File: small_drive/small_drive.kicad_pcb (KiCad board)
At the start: 2 copper layers, 83.8 x 71.8 mm, 146 parts, among them CON1 BARREL_JACK, J1 DB9, M1 SiR826DP, M2 SiR826DP, M3 SiR826DP, M4 SiR826DP, M5 SiR826DP, M6 SiR826DP, M7 SiR826DP, P1 CONN_01X04, P10 CONN_01X02, P11 CONN_01X02, P12 CONN_01X02, P13 CONN_01X04, P14 CONN_01X02, P2 CONN_01X04, P3 CONN_01X06, P4 CONN_01X08, P5 CONN_01X02, P6 CONN_01X02, P7 CONN_01X02, P8 CONN_01X02, P9 CONN_01X04, U1 STM32F334K8, U10 LM5106, U11 ACS711ELCTR-25AB-T, U12 ACS711ELCTR-25AB-T, U13 ACS711ELCTR-25AB-T, U14 STM32F030F4P6TR, U15 LTC2850, U16 LIS3LV02DQ, U17 STM32F030F4P6TR, U18 LTC2850, U19 LIS3LV02DQ, U2 OKR_T3, U20 DS28CM00, U21 DS28CM00, U22 TL431, U23 LT3012, U24 STM32F030F4P6TR, U25 MC33074DTBR2, U3 LTC2850, U4 LTC2850, U5 LTC2850, U6 LT1764EQ, U7 MC33074DTBR2, U8 LM5106, U9 LM5106, Y1 Crystal

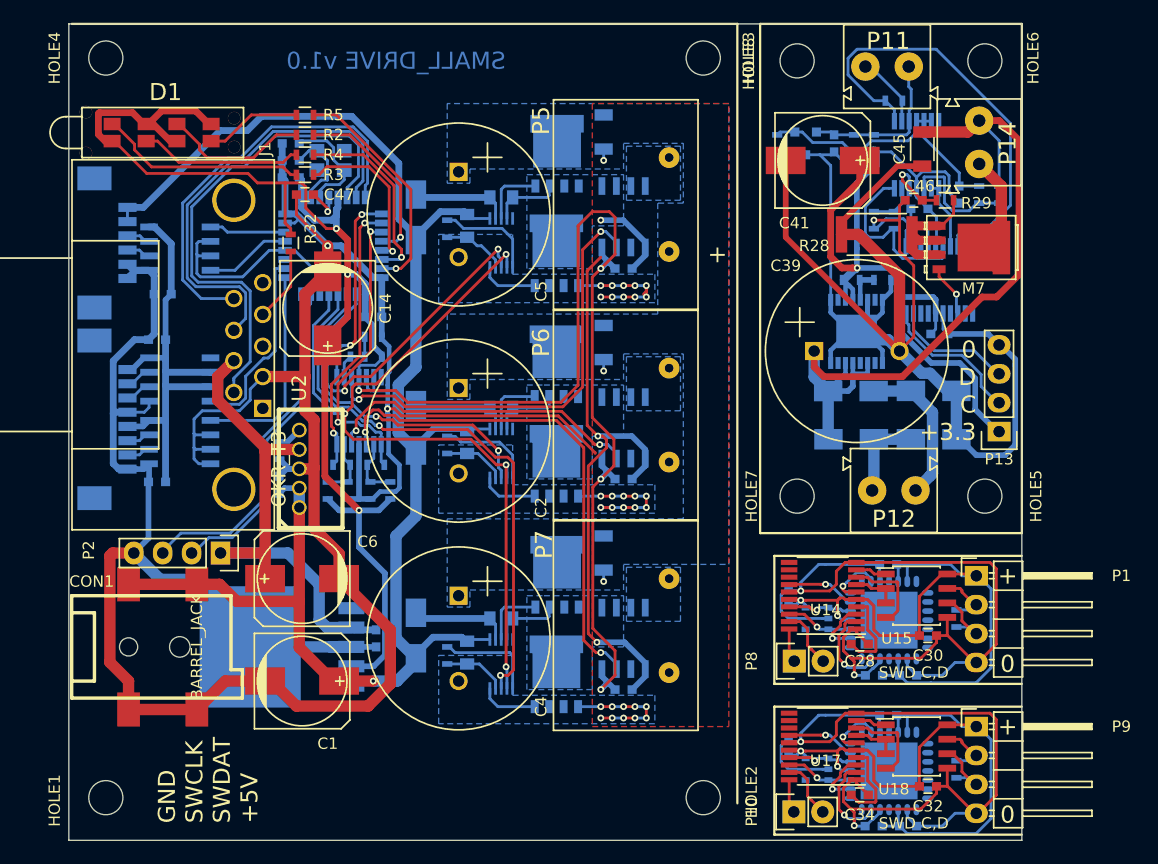
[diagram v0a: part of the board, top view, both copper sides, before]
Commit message: PCB ordered
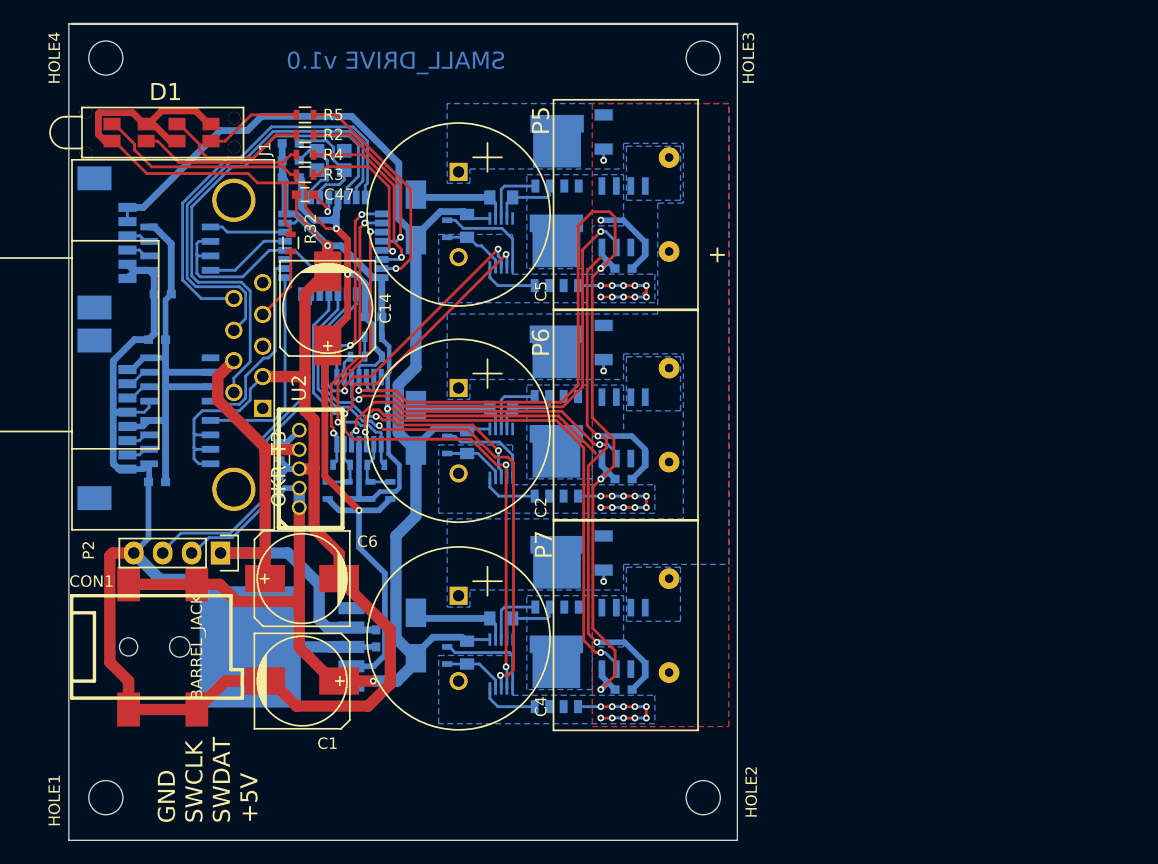
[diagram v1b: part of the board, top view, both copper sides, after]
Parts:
- removed C10, C11, C28, C29, C30, C31, C32, C33, C34, C35, C36, C37, C38, C40, C42, C43, C44: 100nF, Capacitors_SMD:C_0603
- removed C39: 470uF/63V, Capacitors_ThroughHole:C_Radial_D16_L25_P7.5
- removed C41: 100uF/35V, Capacitors_SMD:c_elec_8x10.5
- removed C45: 1uF/100V, Capacitors_SMD:C_1206
- removed C46: C, Capacitors_SMD:C_0603
- removed D5, D6, D7, D8: STPS2150A, Diodes_SMD:SMA_Standard
- removed HOLE5, HOLE6, HOLE7, HOLE8: HOLE, Mounting_Holes:MountingHole_3mm
- removed M7: SiR826DP, 00_Passives:SOT-669_GDS
- removed P1, P9: CONN_01X04, Pin_Headers:Pin_Header_Angled_1x04
- removed P10, P8: CONN_01X02, Pin_Headers:Pin_Header_Straight_1x02
- removed P11, P12, P14: CONN_01X02, 00_Passives:Wiecon_25.197.0253.0
- removed P13: CONN_01X04, Pin_Headers:Pin_Header_Straight_1x04
- removed R18, R19: R, Resistors_SMD:R_0603
- removed R20: 1.5k, Resistors_SMD:R_0603
- removed R21: 300, Resistors_SMD:R_0603
- removed R22: 910, Resistors_SMD:R_0603
- removed R23, R29, R30, R31: 1k, Resistors_SMD:R_0603
- removed R24: 3.0k, Resistors_SMD:R_0603
- removed R25: 1.8k, Resistors_SMD:R_0603
- removed R26: 51k, Resistors_SMD:R_0603
- removed R27: 2.2k, Resistors_SMD:R_0603
- removed R28: R, Resistors_SMD:R_2512
- removed U14, U17, U24: STM32F030F4P6TR, Housings_SSOP:TSSOP-20_4.4x6.5mm_Pitch0.65mm
- removed U15, U18: LTC2850, Housings_SOIC:SOIC-8_3.9x4.9mm_Pitch1.27mm
- removed U16, U19: LIS3LV02DQ, Housings_DFN_QFN:QFN-28-1EP_7x7mm_Pitch0.8mm
- removed U20, U21: DS28CM00, 00_Passives:SOT23_5
- removed U22: TL431, TO_SOT_Packages_SMD:SOT-23
- removed U23: LT3012, Housings_SSOP:TSSOP-16-1EP_4.4x5mm_Pitch0.65mm
- removed U25: MC33074DTBR2, Housings_SSOP:TSSOP-14_4.4x5mm_Pitch0.65mm
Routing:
- net /pomp/Vss: track 169.7 -> 0.00 mm, vias 1 -> 0
- net /pomp/Vdd: track 81.8 -> 0.00 mm, vias 1 -> 0
- net /g_sensor2/Vss: track 79.3 -> 0.00 mm, vias 2 -> 0
- net /g_sensor1/Vss: track 79.3 -> 0.00 mm, vias 2 -> 0
- net /pomp/Vpower: track 69.4 -> 0.00 mm
- net /g_sensor1/Vdd: track 59.6 -> 0.00 mm, vias 2 -> 0
- net /g_sensor2/Vdd: track 59.6 -> 0.00 mm, vias 2 -> 0
- net /pomp/MAINS: track 39.0 -> 0.00 mm
- net /pomp/CURRENT: track 16.0 -> 0.00 mm
- net Net-(C38-Pad1): track 14.3 -> 0.00 mm
- net Net-(D7-PadA): track 13.8 -> 0.00 mm
- net /pomp/SWCLK: track 12.8 -> 0.00 mm
- net Net-(M7-PadS): track 12.5 -> 0.00 mm
- net /pomp/SWDIO: track 10.6 -> 0.00 mm
- net Net-(R26-Pad2): track 10.4 -> 0.00 mm
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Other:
- board size 83.8 x 71.8 mm -> 58.8 x 71.8 mm
- board text removed: "0"
- board text removed: "0 D C +3.3"
- board text removed: "SWD C,D"

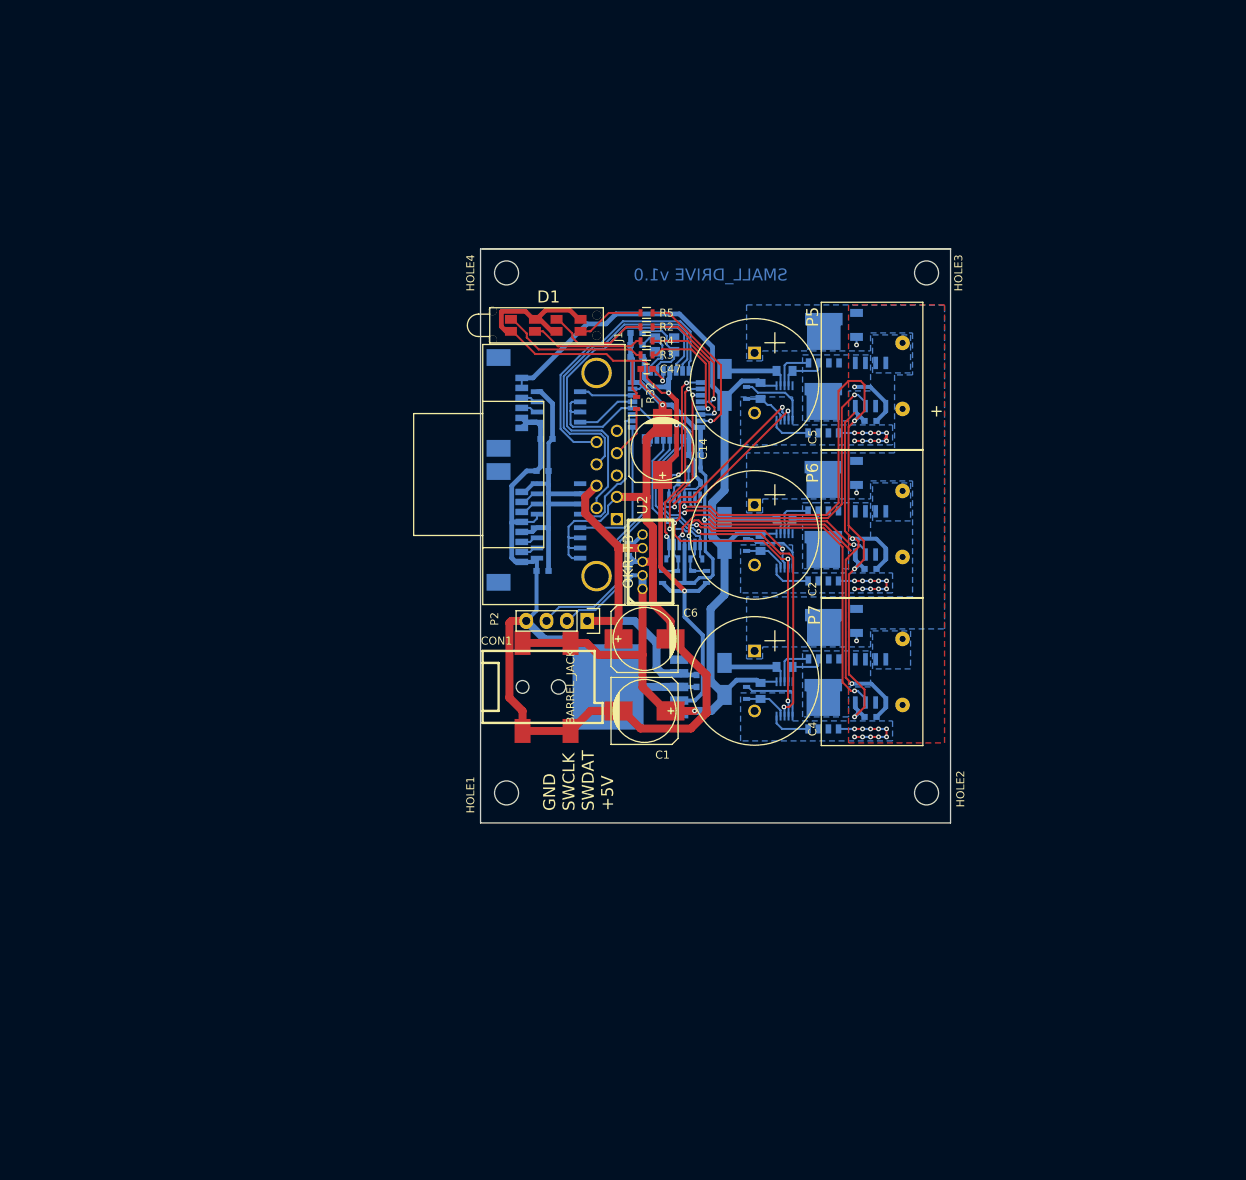
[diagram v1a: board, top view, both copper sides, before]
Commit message: Pauze klus.
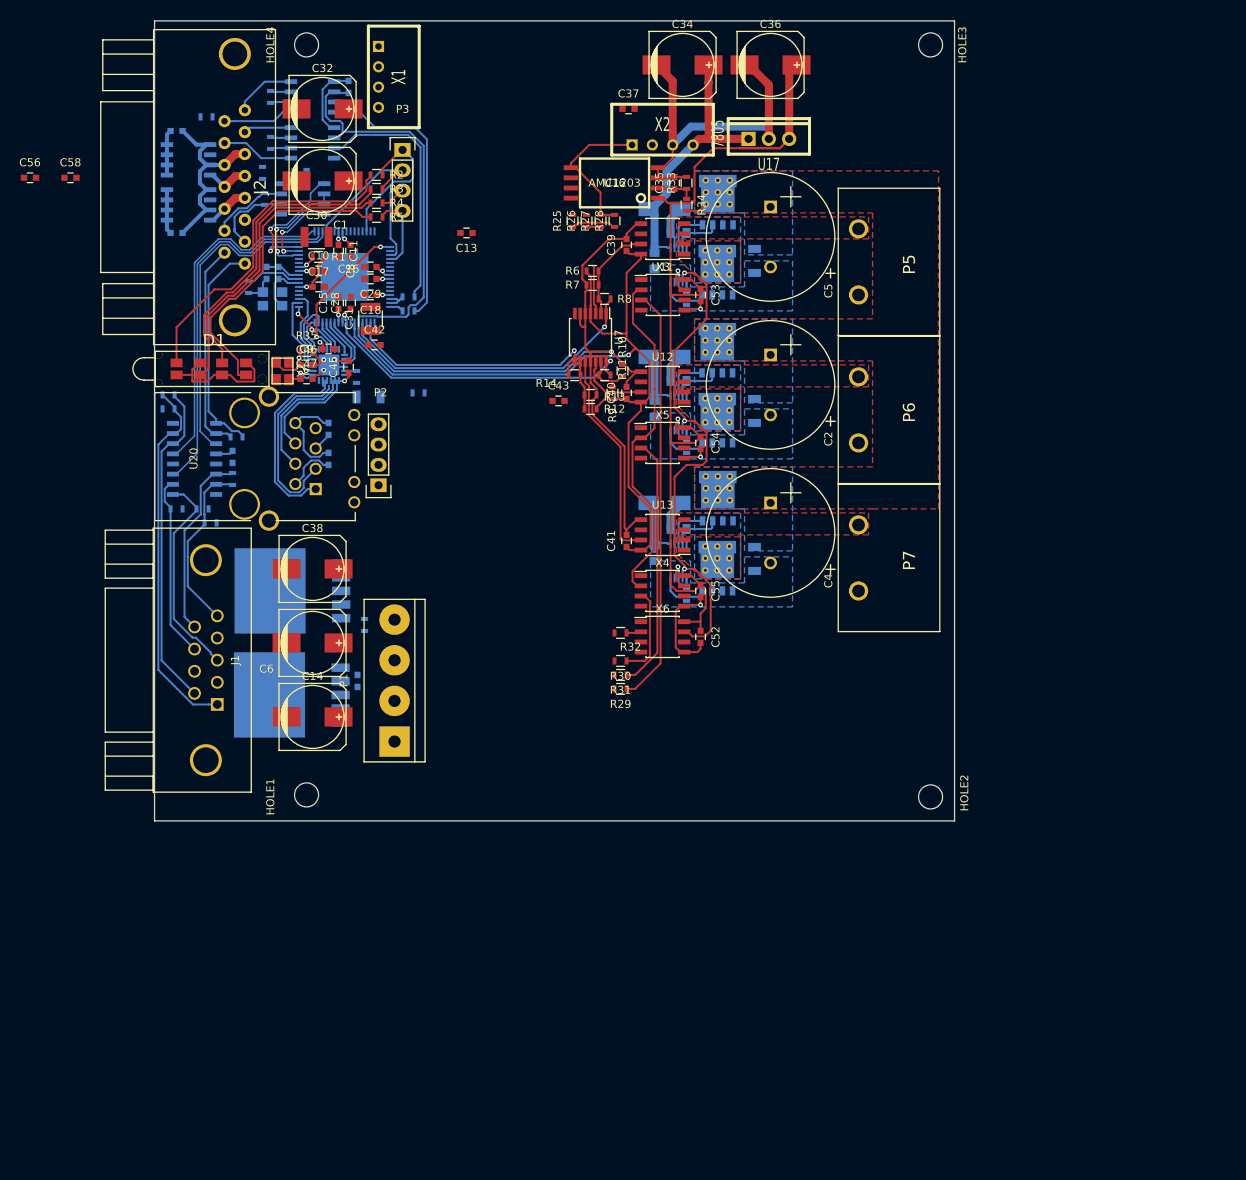
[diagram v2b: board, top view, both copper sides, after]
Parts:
- removed CON1: BARREL_JACK, 00_Passives:smd_barrel_jack
- removed P4: CONN_01X08, Connectors_Molex:Molex_PicoBlade_53261-0871
- added C10: 100nF, Capacitors_SMD:C_0603, F.Cu at (68.5, 79.2)
- added C11: 100nF, Capacitors_SMD:C_0603, F.Cu at (71.0, 76.8)
- added C28: 100nF, Capacitors_SMD:C_0603, F.Cu at (72.5, 83.2)
- added C29: 100nF, Capacitors_SMD:C_0603, F.Cu at (75.0, 80.2)
- added C30: 10uF, Capacitors_SMD:C_1210, F.Cu at (68.2, 75.0)
- added C31: 10uF, Capacitors_SMD:C_1210, F.Cu at (75.0, 85.2)
- added C32: 100uF/35V, Capacitors_SMD:c_elec_8x10.5, F.Cu at (69.0, 59.0)
- added C33: 100nF, Capacitors_SMD:C_0603, B.Cu at (72.2, 56.2)
- added C34: 100uF/35V, Capacitors_SMD:c_elec_8x10.5, F.Cu at (114.0, 53.5)
- added C35: 10nF, Capacitors_SMD:C_0603, F.Cu at (113.0, 68.2)
- added C36: 100uF/35V, Capacitors_SMD:c_elec_8x10.5, F.Cu at (125.0, 53.5)
- added C37: 100nF, Capacitors_SMD:C_0603, F.Cu at (107.2, 59.0)
- added C38: 100uF/35V, Capacitors_SMD:c_elec_8x10.5, F.Cu at (67.8, 116.5)
- added C39: 100nF, Capacitors_SMD:C_0603, F.Cu at (107.0, 76.0)
- added C40: 100nF, Capacitors_SMD:C_0603, F.Cu at (107.0, 94.5)
- added C41: 100nF, Capacitors_SMD:C_0603, F.Cu at (107.0, 113.0)
- added C42: 100nF, Capacitors_SMD:C_0603, F.Cu at (75.5, 88.5)
- added C43: 100nF, Capacitors_SMD:C_0603, F.Cu at (98.5, 95.5)
- added C44: 2.2uF, Capacitors_SMD:C_1206, B.Cu at (74.8, 95.0)
- added C45: 100nF, Capacitors_SMD:C_0603, F.Cu at (72.2, 91.2)
- added C46: 25pF, Capacitors_SMD:C_0603, F.Cu at (67.0, 91.0)
- added C50: 100nF, Capacitors_SMD:C_0603, B.Cu at (69.8, 102.8)
- added C51: 100nF, Capacitors_SMD:C_0603, B.Cu at (69.8, 99.0)
- added C52: 100nF, Capacitors_SMD:C_0603, F.Cu at (116.2, 125.0)
- added C53: 100nF, Capacitors_SMD:C_0603, F.Cu at (116.2, 82.2)
- added C54: 100nF, Capacitors_SMD:C_0603, F.Cu at (116.2, 100.8)
- added C55: 100nF, Capacitors_SMD:C_0603, F.Cu at (116.2, 119.2)
- added C56: 100nF, Capacitors_SMD:C_0603, F.Cu at (32.4, 67.6)
- added C57: 100nF, Capacitors_SMD:C_0603, B.Cu at (57.8, 102.5)
- added C58: 100nF, Capacitors_SMD:C_0603, F.Cu at (37.5, 67.6)
- added C59: 100nF, Capacitors_SMD:C_0603, B.Cu at (66.2, 66.8)
- added J2: DB15, Connectors_Amphenol:DB15F_HD20_SIZE2, F.Cu at (58.0, 68.8)
- added P1: CONN_01X04, Connect:bornier4, F.Cu at (78.0, 130.5)
- added R18: 510, Resistors_SMD:R_0603, B.Cu at (59.8, 81.2)
- added R19: 1k, Resistors_SMD:R_0603, B.Cu at (54.5, 60.0)
- added R20: 1k, Resistors_SMD:R_0603, B.Cu at (61.5, 67.0)
- added R21: R, Resistors_SMD:R_0603, B.Cu at (61.8, 70.2)
- added R22: R, Resistors_SMD:R_0603, B.Cu at (62.5, 57.5)
- added R23: R, Resistors_SMD:R_0603, B.Cu at (62.5, 63.2)
- added R24: R, Resistors_SMD:R_0603, B.Cu at (58.2, 100.0)
- added R25: 1k, Resistors_SMD:R_0603, F.Cu at (100.2, 73.0)
- added R26: 1k, Resistors_SMD:R_0603, F.Cu at (102.0, 73.0)
- added R27: 510, Resistors_SMD:R_0603, F.Cu at (103.8, 73.0)
- added R28: 510, Resistors_SMD:R_0603, F.Cu at (105.5, 73.0)
- added R29: 680, Resistors_SMD:R_0603, F.Cu at (106.2, 131.5)
- added R30: 680, Resistors_SMD:R_0603, F.Cu at (106.2, 128.0)
- added R31: 680, Resistors_SMD:R_0603, F.Cu at (106.2, 129.8)
- added R33: 300, Resistors_SMD:R_0603, F.Cu at (114.5, 68.2)
- added R34: 56k, Resistors_SMD:R_0603, F.Cu at (114.5, 71.0)
- added R35: 6.49k, Resistors_SMD:R_0603, F.Cu at (67.0, 89.2)
- added R36: 220, Resistors_SMD:R_0603, B.Cu at (73.2, 92.5)
- added R37: 220, Resistors_SMD:R_0603, B.Cu at (81.0, 94.5)
- added R38: R, Resistors_SMD:R_0603, B.Cu at (57.8, 105.2)
- added R39: R, Resistors_SMD:R_0603, B.Cu at (50.8, 109.0)
- added R40: R, Resistors_SMD:R_0603, B.Cu at (49.8, 94.8)
- added R41: R, Resistors_SMD:R_0603, B.Cu at (54.0, 109.0)
- added R42: R, Resistors_SMD:R_0603, B.Cu at (55.0, 110.8)
- added R43: R, Resistors_SMD:R_0603, B.Cu at (49.8, 96.5)
- added R44: 22, Resistors_SMD:R_0603, B.Cu at (79.8, 84.2)
- added R45: 22, Resistors_SMD:R_0603, B.Cu at (79.8, 82.5)
- added R46: R, Resistors_SMD:R_0603, B.Cu at (74.2, 123.5)
- added U14: AD8226, Housings_SOIC:SOIC-8_3.9x4.9mm_Pitch1.27mm, B.Cu at (67.8, 63.2)
- added U15: MAX3096, Housings_SOIC:SOIC-16_3.9x9.9mm_Pitch1.27mm, B.Cu at (53.0, 102.8)
- added U16: AMC1203, 00_Passives:SO8_11, F.Cu at (105.5, 68.2)
- added U17: 7805, 00_Local:TO220_78xx, F.Cu at (124.8, 62.8)
- added U18: LT1764EQ, 00_Passives:DD-PAK, B.Cu at (66.2, 119.2)
- added U19: KSZ8081, Housings_DFN_QFN:QFN-24-1EP_4x4mm_Pitch0.5mm, B.Cu at (69.8, 91.0)
- added U20: ETH100_MAG, 00_Passives:ETH100_MAG, F.Cu at (68.1, 106.5)
- added X1: NKE1212DC, 00_Local:NKE-SC, F.Cu at (76.0, 55.0)
- added X2: NKE1212DC, 00_Local:NKE-SC, F.Cu at (111.5, 63.5)
- added X3: HCPL0201, Housings_SOIC:SOIC-8_3.9x4.9mm_Pitch1.27mm, F.Cu at (111.5, 82.2)
- added X4: HCPL0201, Housings_SOIC:SOIC-8_3.9x4.9mm_Pitch1.27mm, F.Cu at (111.5, 119.2)
- added X5: HCPL0201, Housings_SOIC:SOIC-8_3.9x4.9mm_Pitch1.27mm, F.Cu at (111.5, 100.8)
- added X6: HCPL0201, Housings_SOIC:SOIC-8_3.9x4.9mm_Pitch1.27mm, F.Cu at (111.5, 125.0)
- added Y2: 25MHz, Crystals:crystal_FA238-TSX3225, F.Cu at (64.0, 91.8)
- C13, C15, C16, C17, C18, C8, C9, R10, R11, R12, R13, R14, R6, R7, R8, R9, U12, U7: moved to F.Cu
- C47: value 100nF -> 25pF
- C48, C49: value C -> 15pF
- J1: footprint Connect:DB9FC -> Connectors_Amphenol:DB9FC_HD-20
- M1, M2, M3, M4, M5, M6: footprint 00_Passives:SOT-669_GDS -> 00_Passives:SOT-669_GDS_therma
- P3: value CONN_01X06 -> CONN_01X04; footprint Connectors_Molex:Molex_PicoBlade_53261-0671 -> Pin_Headers:Pin_Header_Straight_1x04; moved to F.Cu
- R1: value 270 -> 10k; moved to F.Cu
- R15, R16, R17: value R -> 10k
- R32: value 0 -> 680
- U1: value STM32F334K8 -> XMC4400-F64x512; footprint Housings_QFP:LQFP-32_7x7mm_Pitch0.8mm -> Housings_QFP:LQFP-64-1EP_10x10mm_Pitch0.5mm
- U11, U13: value ACS711ELCTR-25AB-T -> ACS711KLCTR-12AB-T; moved to F.Cu
- U2: value OKR_T3 -> ips511g; footprint 00_Passives:okr_t3 -> Housings_SOIC:SOIC-8_3.9x4.9mm_Pitch1.27mm; moved to B.Cu
- U3: value LTC2850 -> ips511g
- U5: value LTC2850 -> AD8226
- Y1: value Crystal -> 12MHz
- moved C17 87.5 mm to (68.5, 81.2)
- moved C3 79.0 mm to (50.8, 61.8), turned to 0 degrees
- moved C1 77.5 mm to (69.0, 68.0)
- moved U2 72.2 mm to (52.2, 71.0), turned to 180 degrees
- moved C18 71.3 mm to (75.0, 82.2), turned to 180 degrees
- moved C15 68.1 mm to (71.0, 83.2), turned to 90 degrees
- moved U5 63.7 mm to (67.8, 57.5), turned to 0 degrees
- moved C7 62.3 mm to (50.8, 74.5), turned to 0 degrees
- moved U3 55.6 mm to (52.2, 65.4)
- moved C14 55.1 mm to (67.8, 135.0), turned to 0 degrees
- moved J1 53.9 mm to (55.8, 127.9), turned to 270 degrees
- moved R1 53.2 mm to (68.5, 77.5), turned to 180 degrees
- moved C8 50.0 mm to (72.5, 76.8), turned to 270 degrees
- moved Y1 49.3 mm to (62.8, 82.8)
- moved U4 49.3 mm to (66.5, 70.2)
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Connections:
- C19 pad 1: GND -> GNDPWR
- C19 pad 2: +12V -> +12P
- C2 pad 2: GND -> GNDPWR
- C20 pad 1: GND -> GNDPWR
- C20 pad 2: +12V -> +12P
- C21 pad 1: GND -> GNDPWR
- C21 pad 2: +12V -> +12P
- C25 pad 2: GND -> GNDPWR
- C26 pad 2: GND -> GNDPWR
- C27 pad 2: GND -> GNDPWR
- C4 pad 2: GND -> GNDPWR
- C48 pad 1: GND -> Net-(C48-Pad1)
- C48 pad 2: Net-(C48-Pad2) -> GND
- C5 pad 2: GND -> GNDPWR
- C9 pad 1: +5V -> +3.3V
- D2 pad A: +12V -> +12P
- D3 pad A: +12V -> +12P
- D4 pad A: +12V -> +12P
- M2 pad S: GND -> GNDPWR
- M4 pad S: GND -> GNDPWR
- M6 pad S: GND -> GNDPWR
- P2 pad 1: +5V -> +3.3V
- P2 pad 2: /SWDAT -> Net-(P2-Pad2)
- P2 pad 3: /SWCLK -> Net-(P2-Pad3)
- P3 pad 1: GND -> /LED0
- P3 pad 2: GND -> /LED1
- P3 pad 3: Net-(P3-Pad3) -> /LED2
- P3 pad 4: Net-(P3-Pad4) -> /LED3
- P5 pad 1: +60V -> /M0
- P5 pad 2: /M0 -> +60V
- P6 pad 1: GND -> /M1
- P6 pad 2: /M1 -> GNDPWR
- P7 pad 1: GND -> /M2
- P7 pad 2: /M2 -> GNDPWR
- R1 pad 1: Net-(R1-Pad1) -> +3.3V
- R1 pad 2: GND -> Net-(R1-Pad2)
- R12 pad 1: +3.3V -> +3.3VADC
- R15 pad 2: GND -> GNDPWR
- R16 pad 2: GND -> GNDPWR
- R17 pad 2: GND -> GNDPWR
- R2 pad 1: Net-(D1-Pad6) -> Net-(D1-Pad8)
- R3 pad 1: Net-(D1-Pad8) -> Net-(D1-Pad2)
- R32 pad 1: +3.3V -> Net-(R32-Pad1)
- R32 pad 2: Net-(J1-Pad4) -> /HBEN
- R4 pad 1: Net-(D1-Pad2) -> Net-(D1-Pad6)
- R6 pad 1: +3.3V -> +3.3VADC
- R9 pad 1: +3.3V -> +3.3VADC
- U1 pad 1: +3.3V -> /ETH_CRS_DVA
- U1 pad 10: /CUR1 -> Net-(U1-Pad10)
- U1 pad 11: /CUR2 -> Net-(U1-Pad11)
- U1 pad 12: /LED0 -> Net-(U1-Pad12)
- U1 pad 13: /LED1 -> +3.3V
- U1 pad 14: /LED2 -> /ENC_SIN
- U1 pad 15: /LED3 -> /ENC_SIN
- U1 pad 16: GND -> /ENC_COS
- U1 pad 17: +3.3V -> Net-(U1-Pad17)
- U1 pad 18: /HB0 -> /CUR2
- U1 pad 19: /HB1 -> Net-(U1-Pad19)
- U1 pad 2: Net-(C48-Pad2) -> /ENC_RXD2
- U1 pad 20: /HB2 -> /CUR0
- U1 pad 21: /HBEN -> GND
- U1 pad 22: /DXD -> +3.3VADC
- U1 pad 23: /SWDAT -> Net-(U1-Pad23)
- U1 pad 24: /SWCLK -> /CUR1
- U1 pad 25: /ENC_RXD -> /VddC
- U1 pad 26: /ENC_TXD -> +3.3V
- U1 pad 27: Net-(U1-Pad27) -> /ETH0_TXD1
- U1 pad 28: /DXD -> /ETH0_TXD0
- U1 pad 29: /TXD -> /ETH0_TX_EN
- U1 pad 3: Net-(C49-Pad2) -> /LED2
- U1 pad 30: /RXD -> /ETH0_RXERA
- U1 pad 31: GND -> /ETH0_RXD1A
- U1 pad 32: GND -> /ETH0_RXD0A
- U1 pad 4: Net-(C47-Pad1) -> /LED3
- U1 pad 5: +3.3V -> Net-(U1-Pad5)
- U1 pad 6: /A -> Net-(U1-Pad6)
- U1 pad 7: /B -> Net-(U1-Pad7)
- U1 pad 8: /Z -> +3.3V
- U1 pad 9: /CUR0 -> /VddC
- U10 pad 1: +12V -> +12P
- U10 pad 7: /HBEN -> Net-(U10-Pad7)
- U10 pad 8: /HB2 -> Net-(U10-Pad8)
- U10 pad 9: GND -> GNDPWR
- U11 pad 8: +3.3V -> +3.3VADC
- U12 pad 8: +3.3V -> +3.3VADC
- U13 pad 8: +3.3V -> +3.3VADC
- U2 pad 1: +12V -> GND
- U2 pad 2: +12V -> /ENC_5V
- U2 pad 4: +5V -> Net-(J2-Pad11)
- U2 pad 5: Net-(R1-Pad1) -> +5V
- U3 pad 1: /RXD -> GND
- U3 pad 2: /DXD -> /ENC_12V
- U3 pad 3: /DXD -> GND
- U3 pad 4: /TXD -> Net-(J2-Pad12)
- U3 pad 5: GND -> +12V
- U3 pad 6: Net-(P3-Pad3) -> +12V
- U3 pad 7: Net-(P3-Pad4) -> +12V
- U3 pad 8: +5V -> +12V
- U4 pad 1: Net-(U4-Pad1) -> /ENC_RXD
- U4 pad 2: +5V -> /ENC_DIR
- U4 pad 3: +5V -> /ENC_DIR
- U4 pad 8: +5V -> +3.3V
- U5 pad 1: /ENC_RXD -> Net-(J2-Pad15)
- U5 pad 2: GND -> Net-(R22-Pad1)
- U5 pad 3: GND -> Net-(R22-Pad2)
- U5 pad 4: GND -> Net-(J2-Pad8)
- U5 pad 5: GND -> -12V
- U5 pad 6: Net-(P4-Pad2) -> GND
- U5 pad 8: +5V -> +12V
- U6 pad 1: Net-(U6-Pad1) -> +5V
- U7 pad 4: +3.3V -> +3.3VADC
- U8 pad 1: +12V -> +12P
- U8 pad 7: /HBEN -> Net-(U10-Pad7)
- U8 pad 8: /HB0 -> Net-(U8-Pad8)
- U8 pad 9: GND -> GNDPWR
- U9 pad 1: +12V -> +12P
- U9 pad 7: /HBEN -> Net-(U10-Pad7)
- U9 pad 8: /HB1 -> Net-(U9-Pad8)
- U9 pad 9: GND -> GNDPWR
- Y1 pad 1: Net-(C48-Pad2) -> Net-(C48-Pad1)
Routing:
- net GND: track 369.6 -> 222.9 mm, vias 38 -> 4
- net +3.3V: track 216.0 -> 77.8 mm, vias 7 -> 6
- net +12V: track 143.8 -> 5.71 mm, vias 1 -> 0
- net +5P: track 0.00 -> 115.9 mm
- net +3.3VADC: track 0.00 -> 105.0 mm, vias 0 -> 1
- net +5V: track 89.2 -> 5.59 mm
- net /HBEN: track 72.6 -> 0.00 mm, vias 4 -> 0
- net GNDPWR: track 0.00 -> 65.5 mm, vias 0 -> 3
- net Net-(U10-Pad7): track 0.00 -> 63.7 mm, vias 0 -> 3
- net Net-(R29-Pad1): track 0.00 -> 52.3 mm
- net +12P: track 0.00 -> 50.6 mm
- net /HB2: track 49.7 -> 0.00 mm, vias 2 -> 0
- net /~A: track 0.00 -> 46.9 mm
- net /ENC_B: track 0.00 -> 46.2 mm
- net /ENC_A: track 0.00 -> 43.0 mm
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- added copper zone on F.Cu, net +60V
- added copper zone on F.Cu, net /M0
- added copper zone on F.Cu, net /M1
- added copper zone on F.Cu, net /M2
- added copper zone on F.Cu, net /SW0
- added copper zone on F.Cu, net /SW1
- added copper zone on F.Cu, net /SW2
- added copper zone on B.Cu, net GNDPWR
- removed copper zone on B.Cu, net /M0
- removed copper zone on B.Cu, net /M1
- removed copper zone on B.Cu, net /M2
- removed copper zone on B.Cu, net GND
- removed copper zone on F.Cu, net GND
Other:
- board size 58.8 x 71.8 mm -> 100 x 100 mm
- board text removed: "GND SWCLK SWDAT +5V"
- board text removed: "SMALL_DRIVE v1.0"
